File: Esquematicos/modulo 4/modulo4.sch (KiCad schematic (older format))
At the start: 23 parts, among them P1 CONN_10X2, P2 CONN_10X2, P3 batt, U1 MINI_USB, U2 TPS63002, U3 TPS63001

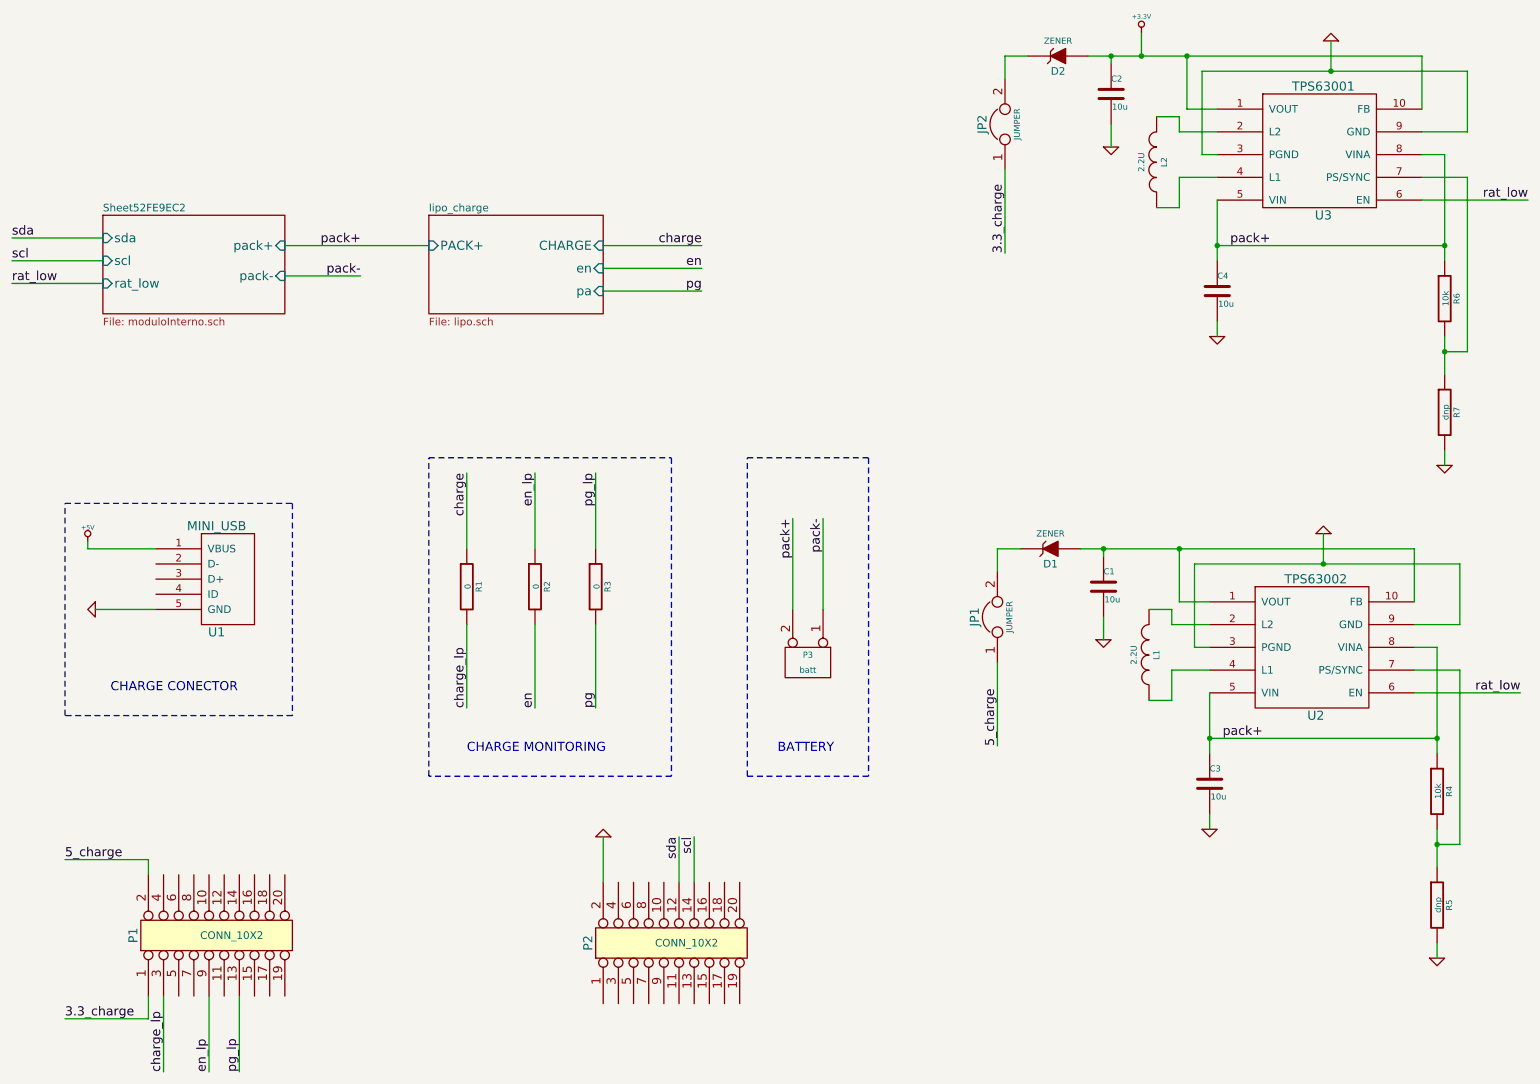
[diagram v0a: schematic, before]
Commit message: recuperacion
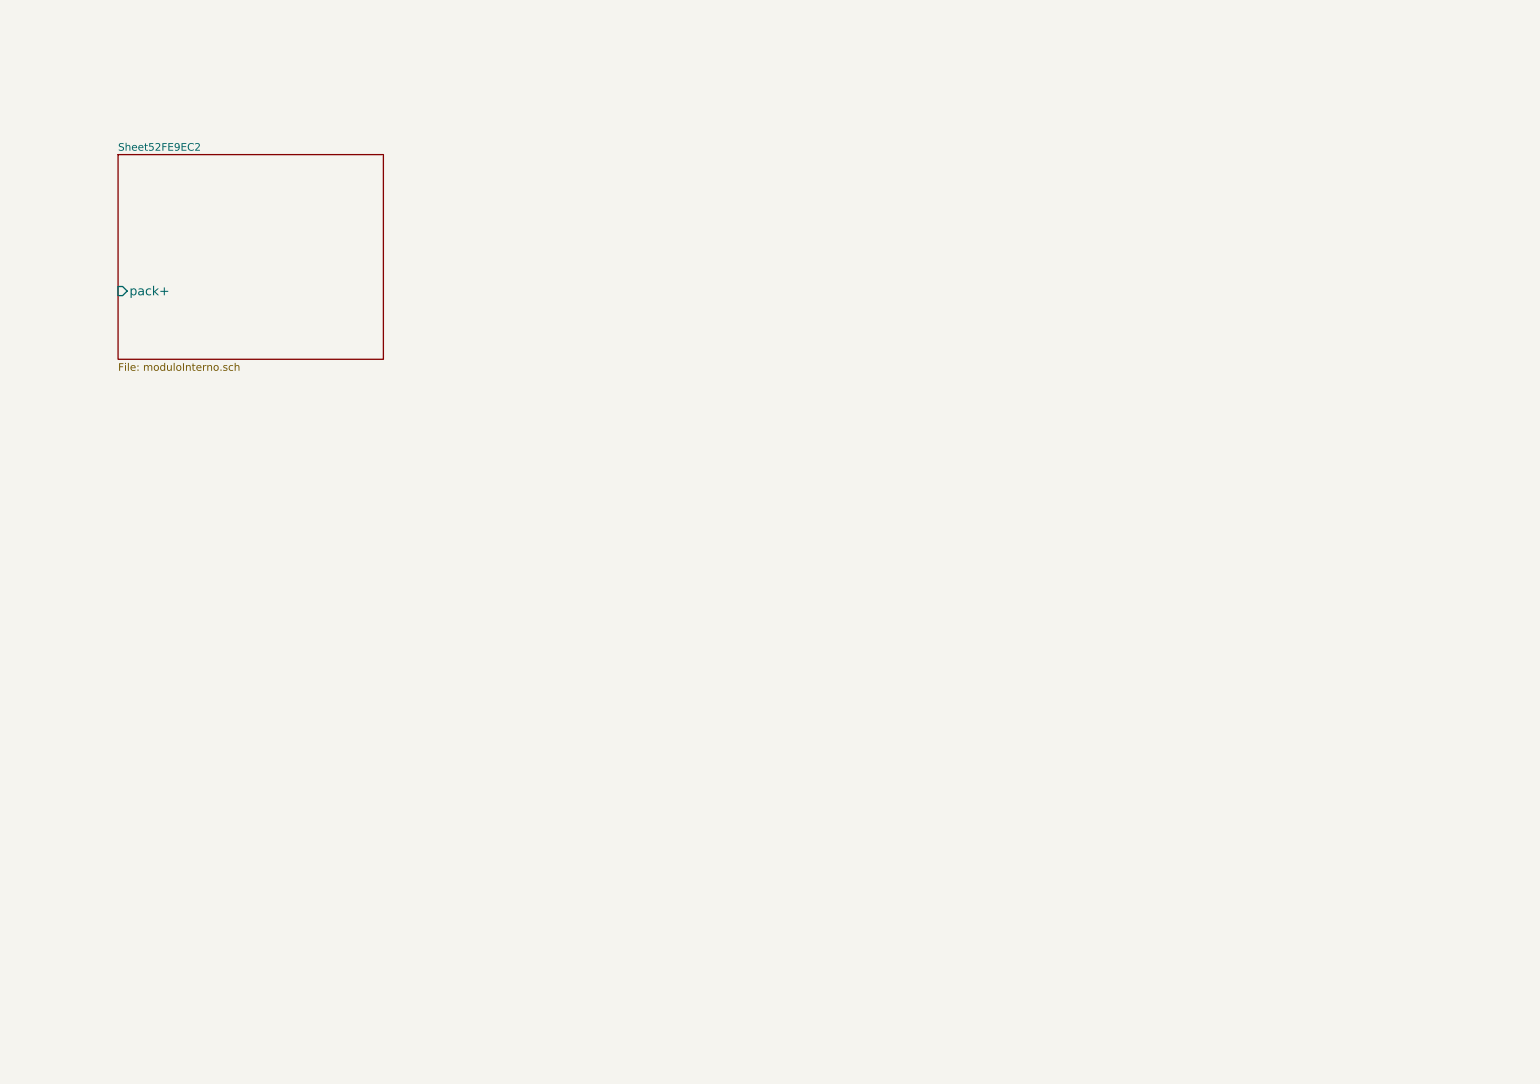
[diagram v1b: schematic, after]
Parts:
- removed C1, C2, C3, C4: 10u, ~, symbol C
- removed D1, D2: ZENER, ~, symbol ZENER
- removed JP1, JP2: JUMPER, ~, symbol JUMPER
- removed L1, L2: 2.2U, ~, symbol INDUCTOR
- removed P1, P2: CONN_10X2, symbol CONN_10X2
- removed P3: batt, symbol CONN_2
- removed R1, R2, R3: 0, ~, symbol R
- removed R4, R6: 10k, ~, symbol R
- removed R5, R7: dnp, ~, symbol R
- removed U1: MINI_USB, ~, symbol MINI_USB
- removed U2: TPS63002, ~, symbol TPS63002
- removed U3: TPS63001, ~, symbol TPS63001
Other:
- note removed: "BATTERY\n"
- note removed: "CHARGE CONECTOR"
- note removed: "CHARGE MONITORING"
